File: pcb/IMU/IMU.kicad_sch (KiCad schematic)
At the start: 12 parts, among them J1 Pin Bus, U1 ICM-20948, U3 MIC5365-1.8YC5

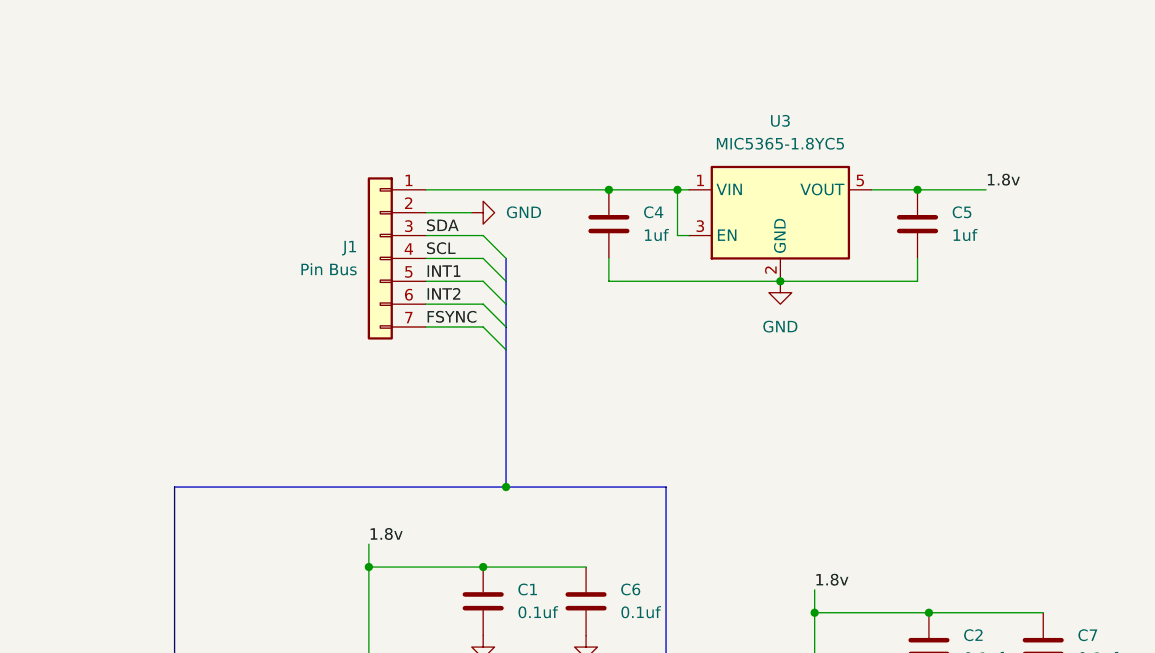
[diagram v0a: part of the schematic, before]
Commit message: updated pcb
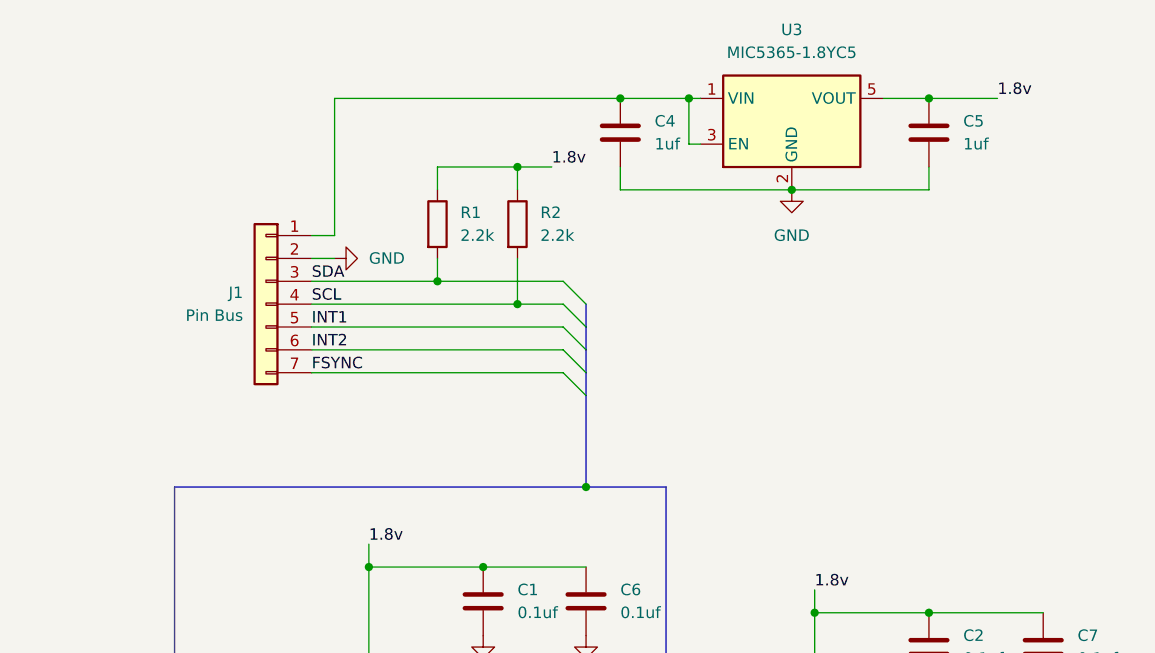
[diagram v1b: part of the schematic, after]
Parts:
- added R1, R2: 2.2k, Resistor_SMD:R_0603_1608Metric_Pad0.98x0.95mm_HandSolder, symbol Device:R
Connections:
- net 1.8v: now also R1.1, R2.1
- net SCL: now also R2.2
- net SDA: now also R1.2
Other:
- moved on the sheet: C4, C5, J1, U3

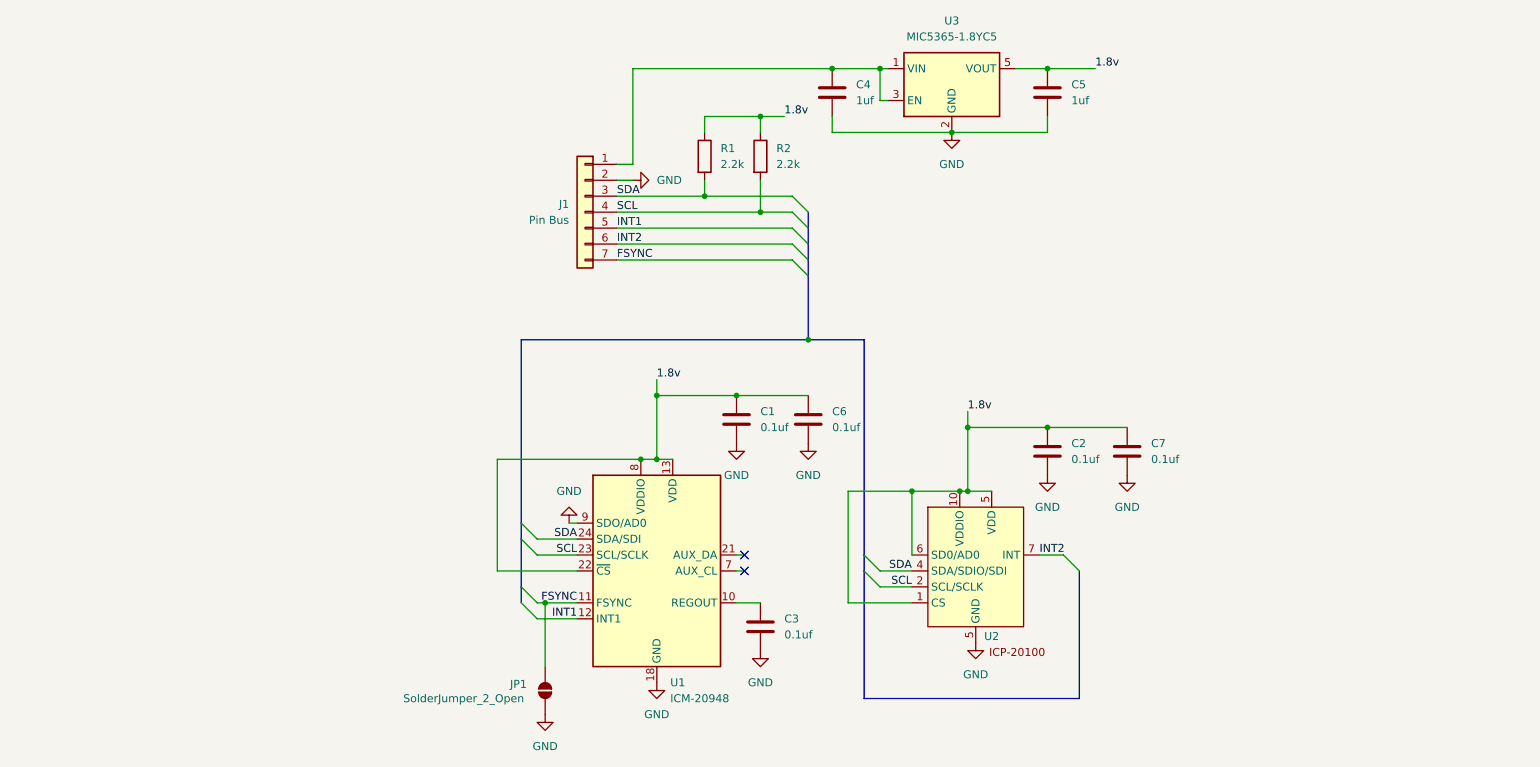
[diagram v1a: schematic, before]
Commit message: IMU v0.5
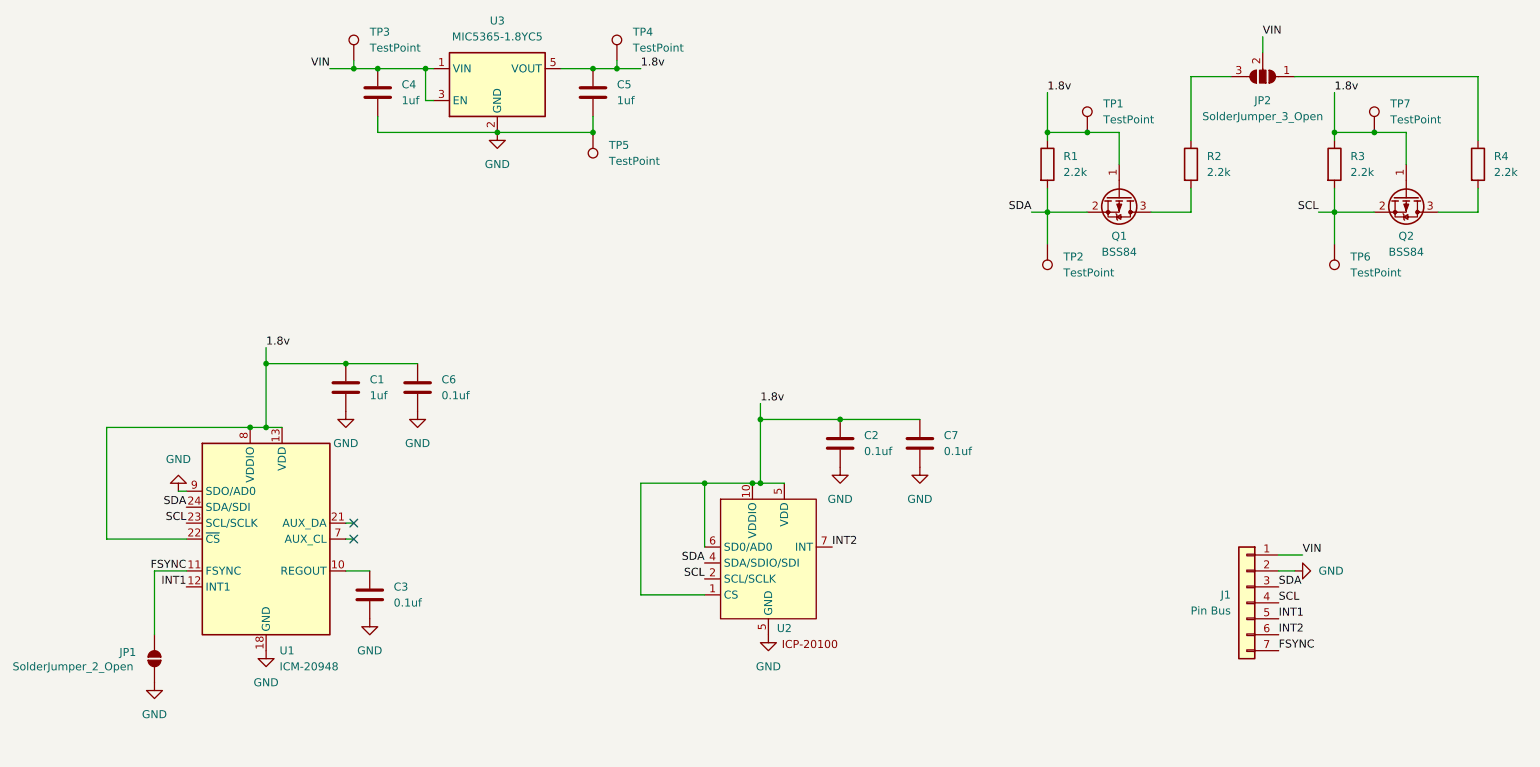
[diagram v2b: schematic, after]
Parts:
- added JP2: SolderJumper_3_Open, Jumper:SolderJumper-3_P1.3mm_Open_Pad1.0x1.5mm, symbol Jumper:SolderJumper_3_Open
- added Q1, Q2: BSS84, Package_TO_SOT_SMD:SOT-23, symbol Transistor_FET:BSS84
- added R3, R4: 2.2k, Resistor_SMD:R_0603_1608Metric_Pad0.98x0.95mm_HandSolder, symbol Device:R
- added TP1, TP2, TP3, TP4, TP5, TP6, TP7: TestPoint, TestPoint:TestPoint_Pad_D1.0mm, symbol Connector:TestPoint
- C1: value 0.1uf -> 1uf; footprint Capacitor_SMD:C_0402_1005Metric_Pad0.74x0.62mm_HandSolder -> Capacitor_SMD:C_0603_1608Metric_Pad1.08x0.95mm_HandSolder
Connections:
- net 1.8v: now also Q1.1 (G), Q2.1 (G), R3.1, TP1.1, TP4.1, TP7.1; no longer R2.1
- net GND: now also TP5.1
- net SCL: now also Q2.2 (S), R3.2, TP6.1; no longer R2.2
- net SDA: now also Q1.2 (S), TP2.1
- net VIN: now reaches C4.1, J1.1 (Pin_1), U3.1 (VIN), U3.3 (EN)
- net VIN: now also JP2.2 (C), TP3.1
- new net: Q2.3 (D), R4.2
- new net: JP2.3 (B), R2.1
- new net: Q1.3 (D), R2.2
- new net: JP2.1 (A), R4.1
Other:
- moved on the sheet: C1, C2, C3, C4, C5, C6, C7, J1, JP1, U1, U2, U3
